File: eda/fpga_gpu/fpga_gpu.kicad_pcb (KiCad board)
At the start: 2 copper layers, 94.5 x 68.3 mm, 57 parts, among them J1 VGA, J2 Bus expansion, U1 ICE40HX4K-TQ144, U2 SST25VF080B-50-4x-S2Ax, U3 74HCT541, U4 74HCT541, U5 74HCT541, U6 TXS0108EPW, U7 TXS0108EPW, U8 AMS1117-3.3, U9 AP2112K-1.2, X1 TXC-7C

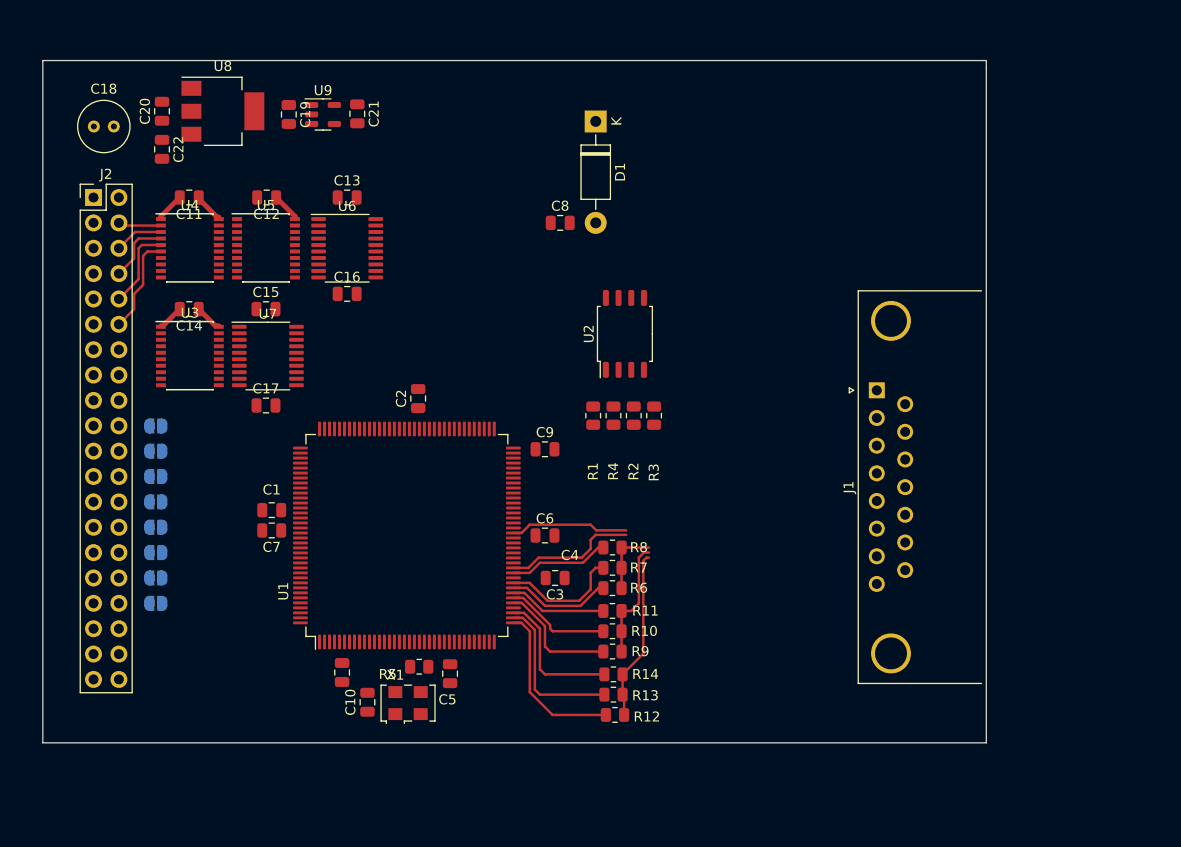
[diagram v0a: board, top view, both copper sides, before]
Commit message: GPU routing
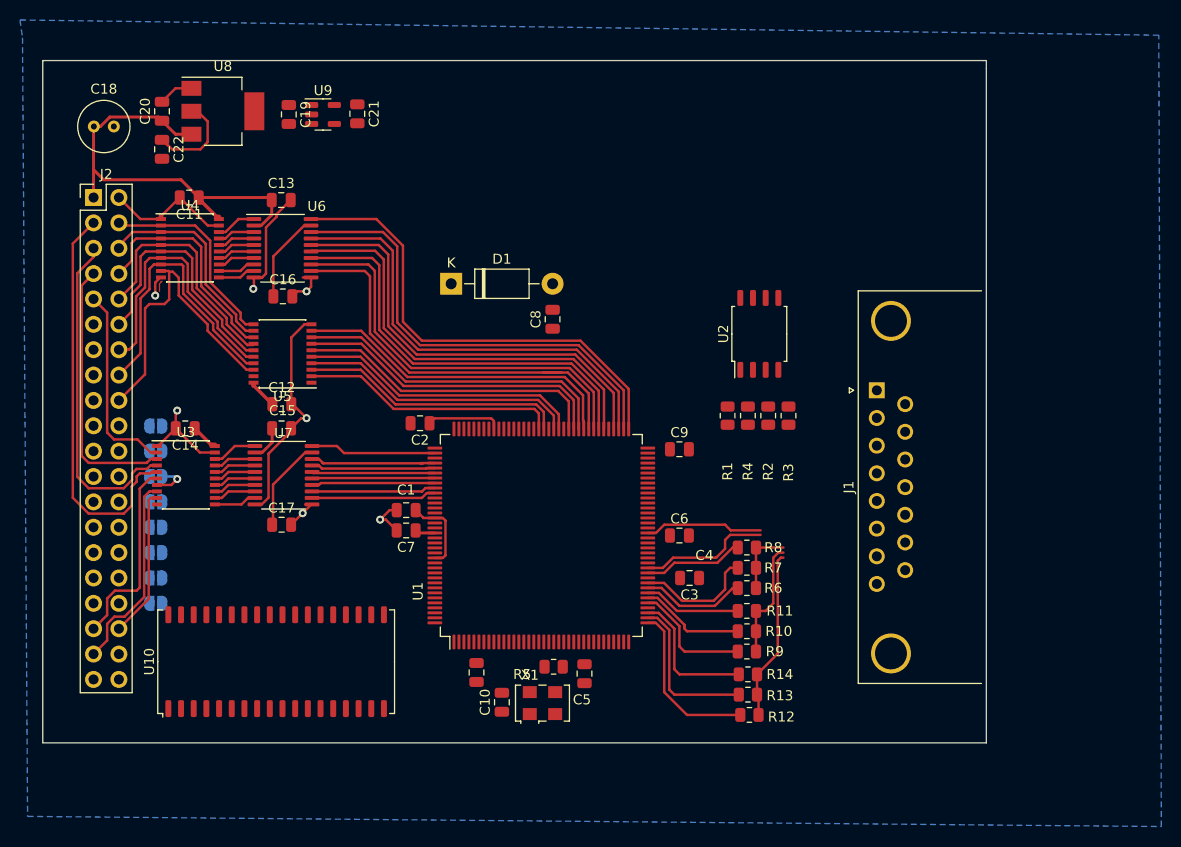
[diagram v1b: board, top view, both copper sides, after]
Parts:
- added U10: IS61C5128AL-10KLI, Package_SO:SOJ-36_10.16x23.49mm_P1.27mm, F.Cu at (43.2, 106.4)
- moved D1 21.8 mm to (60.7, 68.6), turned to 0 degrees
- moved C12 20.8 mm to (43.7, 80.6), turned to 0 degrees
- moved C1 13.5 mm to (56.2, 91.3)
- moved C10 13.5 mm to (65.8, 110.5)
- moved C4 13.5 mm to (63.2, 107.5)
- moved C5 13.5 mm to (74.1, 107.6)
- moved C6 13.5 mm to (83.6, 93.8)
- moved C7 13.5 mm to (56.2, 93.3)
- moved C9 13.5 mm to (83.6, 85.2)
- moved R12 13.5 mm to (90.6, 111.8)
- moved R13 13.5 mm to (90.4, 109.7)
- moved R14 13.5 mm to (90.4, 107.7)
- moved R2 13.5 mm to (92.5, 81.8)
- moved R3 13.5 mm to (94.5, 81.8)
- moved R4 13.5 mm to (90.4, 81.8)
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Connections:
- U1 pad 110: /Interfacing/ADev0 -> /Interfacing/ADev3
- U1 pad 112: /Interfacing/ADev1 -> /Interfacing/ADev2
- U1 pad 113: /Interfacing/ADev2 -> /Interfacing/ADev1
- U1 pad 114: /Interfacing/ADev3 -> /Interfacing/ADev0
- U3 pad 2: /Interfacing/Expansion/A0 -> /Interfacing/Expansion/A3
- U3 pad 3: /Interfacing/Expansion/A1 -> /Interfacing/Expansion/A2
- U3 pad 4: /Interfacing/Expansion/A2 -> /Interfacing/Expansion/A1
- U3 pad 5: /Interfacing/Expansion/A3 -> /Interfacing/Expansion/A0
- U5 pad 11: /Interfacing/Expansion/D7 -> /Interfacing/Expansion/D0
- U5 pad 12: /Interfacing/Expansion/D6 -> /Interfacing/Expansion/D1
- U5 pad 13: /Interfacing/Expansion/D5 -> /Interfacing/Expansion/D2
- U5 pad 14: /Interfacing/Expansion/D4 -> /Interfacing/Expansion/D3
- U5 pad 15: /Interfacing/Expansion/D3 -> /Interfacing/Expansion/D4
- U5 pad 16: /Interfacing/Expansion/D2 -> /Interfacing/Expansion/D5
- U5 pad 17: /Interfacing/Expansion/D1 -> /Interfacing/Expansion/D6
- U5 pad 18: /Interfacing/Expansion/D0 -> /Interfacing/Expansion/D7
- U5 pad 2: /DOut0 -> /DOut7
- U5 pad 3: /DOut1 -> /DOut6
- U5 pad 4: /DOut2 -> /DOut5
- U5 pad 5: /DOut3 -> /DOut4
- U5 pad 6: /DOut4 -> /DOut3
- U5 pad 7: /DOut5 -> /DOut2
- U5 pad 8: /DOut6 -> /DOut1
- U5 pad 9: /DOut7 -> /DOut0
- U7 pad 16: /Interfacing/ADev3 -> /Interfacing/ADev0
- U7 pad 17: /Interfacing/ADev2 -> /Interfacing/ADev1
- U7 pad 18: /Interfacing/ADev1 -> /Interfacing/ADev2
- U7 pad 20: /Interfacing/ADev0 -> /Interfacing/ADev3
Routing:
- net GND: track 5.31 -> 73.2 mm, vias 0 -> 7
- net /DIn0: track 0.00 -> 47.3 mm
- net /DIn1: track 0.00 -> 46.2 mm
- net /DIn2: track 0.00 -> 45.2 mm
- net VCC: track 8.34 -> 52.7 mm
- net /DIn3: track 0.00 -> 44.3 mm
- net +3.3V: track 0.00 -> 43.4 mm
- net /DIn4: track 0.00 -> 43.1 mm
- net /DIn7: track 0.00 -> 42.3 mm
- net /DIn5: track 0.00 -> 41.9 mm
- net /DIn6: track 0.00 -> 40.9 mm
- net /Interfacing/Expansion/A0: track 0.00 -> 40.6 mm
- net /Interfacing/Expansion/A1: track 0.00 -> 33.3 mm
- net /DOut0: track 0.00 -> 33.3 mm
- net /DOut1: track 0.00 -> 32.4 mm
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- added copper zone on B.Cu, net GND
